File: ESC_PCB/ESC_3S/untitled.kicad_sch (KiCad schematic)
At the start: 15 parts, among them J4 Conn_01x04_Pin, U5 SN65HVD230DR

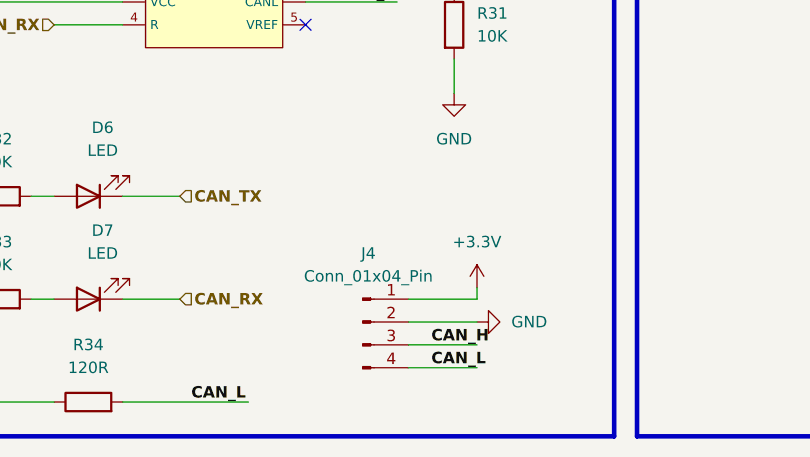
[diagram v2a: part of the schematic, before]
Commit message: layout
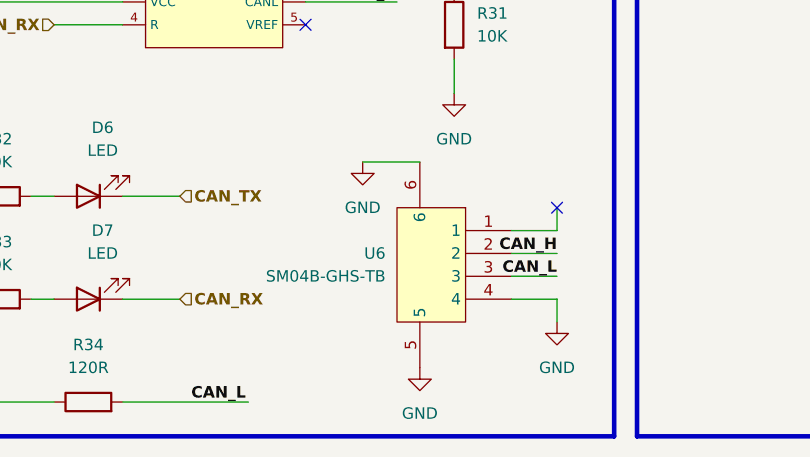
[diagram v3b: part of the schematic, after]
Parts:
- removed J4: Conn_01x04_Pin, Connector_PinHeader_2.54mm:PinHeader_1x04_P2.54mm_Vertical, symbol Connector:Conn_01x04_Pin
- added U6: SM04B-GHS-TB, easyeda2kicad:CONN-SMD_4P-P1.25_SM04B-GHS-TB-LF-SN, symbol easyeda2kicad:SM04B-GHS-TB
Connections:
- net CAN_H: now also U6.2
- net CAN_L: now also U6.3
- net GND: now also U6.4, U6.5, U6.6
- no-connect marks 1 -> 2
